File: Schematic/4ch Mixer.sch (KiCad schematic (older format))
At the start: 44 parts, among them J1 3.5mm_Mono_Jack_With_Switch, J2 3.5mm_Mono_Jack_With_Switch, J3 3.5mm_Mono_Jack_With_Switch, J4 3.5mm_Mono_Jack_With_Switch, J5 3.5mm_Mono_Jack_With_Switch, J6 3.5mm_Mono_Jack_With_Switch, P1 CONN_02X08, U1 TL074, U2 TL072

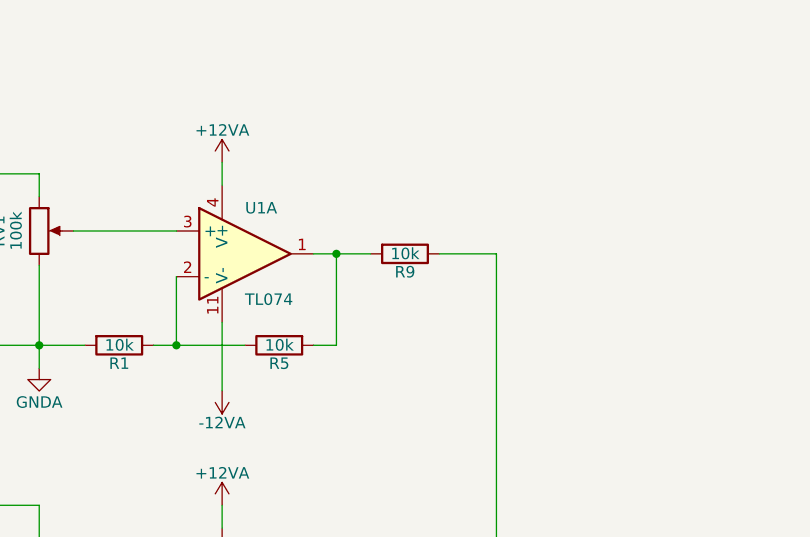
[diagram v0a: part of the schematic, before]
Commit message: I think the board is done
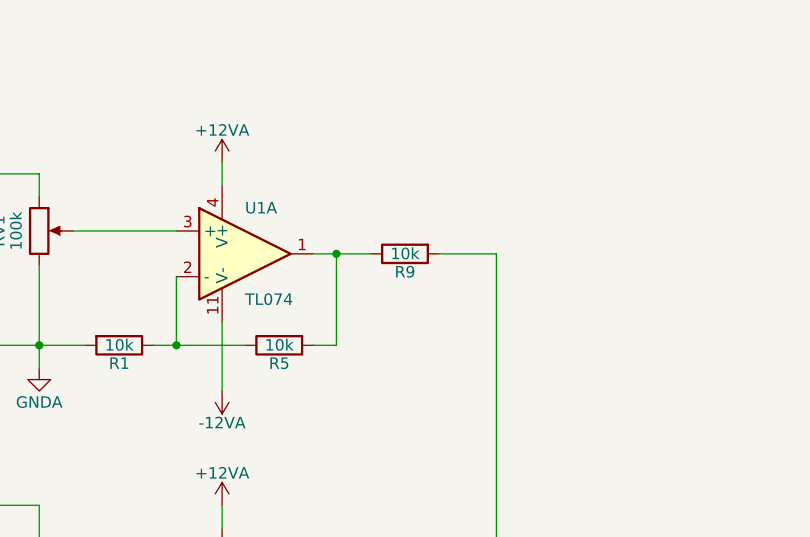
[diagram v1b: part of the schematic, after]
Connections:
- net at R5.2, U1.1: now also R9.1; no longer R9.2
- net at R10.1, R11.1, R12.1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: now also R9.2; no longer R9.1
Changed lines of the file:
@@
 F 3 "" H 3800 1600 50  0000 C CNN
 	1    3800 1600
-	0    1    1    0
+	0    -1   1    0
 $EndComp
 $Comp
